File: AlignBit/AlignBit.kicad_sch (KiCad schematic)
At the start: 8 parts, among them J1 Conn_01x04_Pin, U1 STM32C011J_4-6_Mx, U4 VL53L0CXV0DH_1, U5 VL53L0CXV0DH_1, U6 VL53L0CXV0DH_1, U7 VL53L0CXV0DH_1

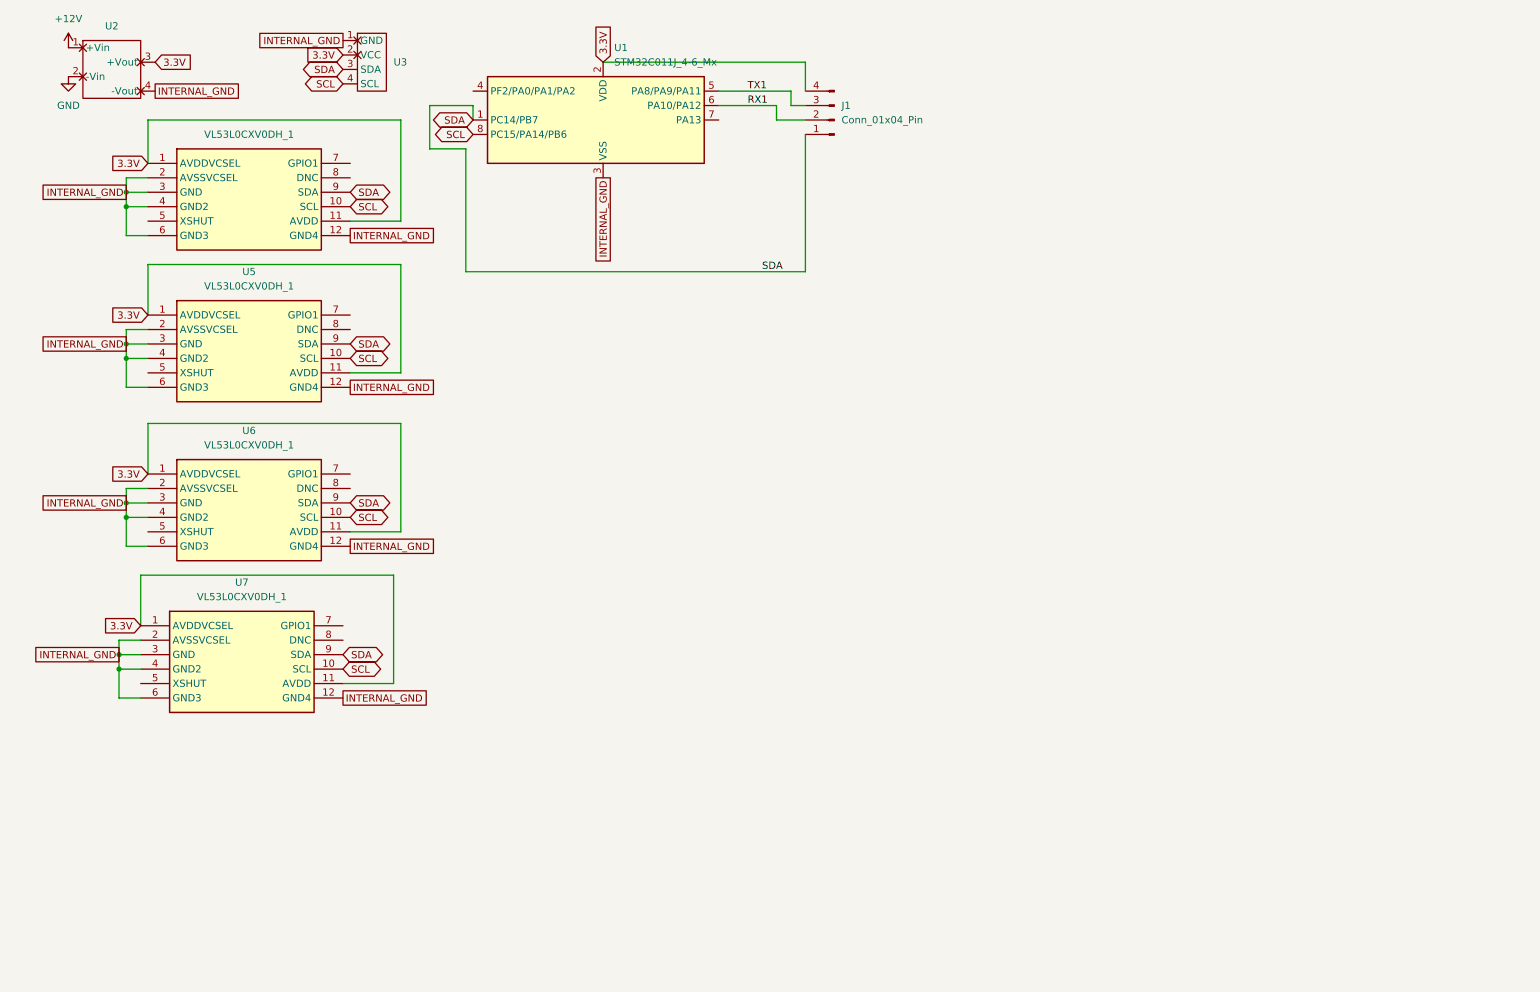
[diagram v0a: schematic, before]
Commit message: Adding things untill its done
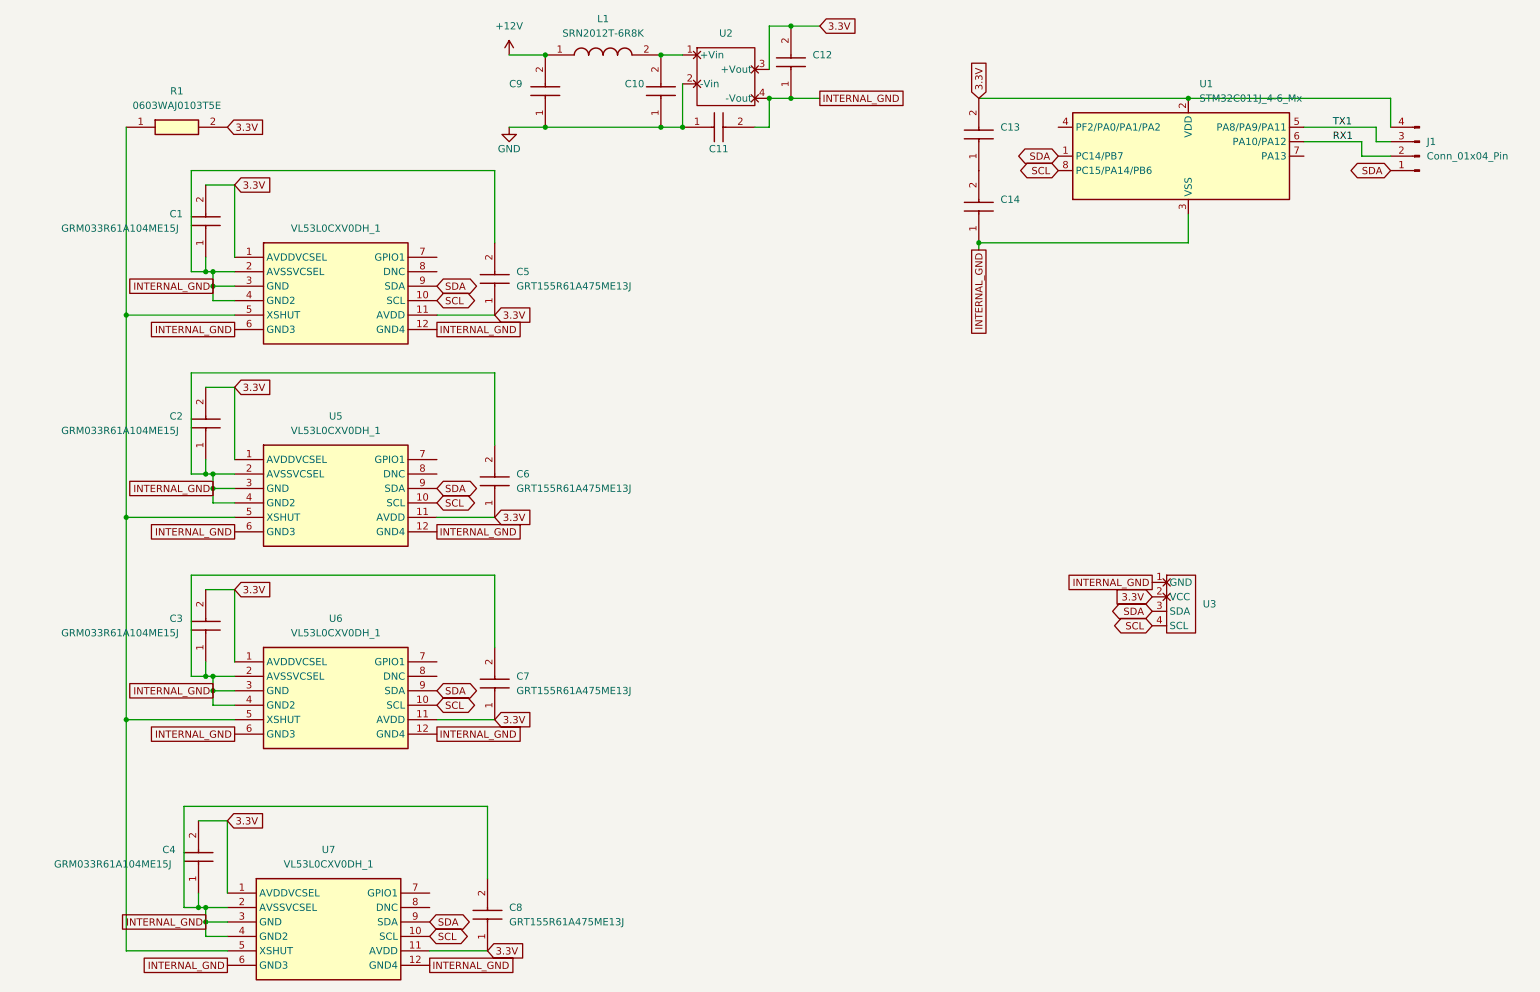
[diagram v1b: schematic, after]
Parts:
- added C1, C10, C13, C2, C3, C4, C9: GRM033R61A104ME15J, CAPC0603X33N, symbol GRM033R61A104ME15J:GRM033R61A104ME15J
- added C11: C0402C271K5RAC, CAPC1005X55N, symbol C0402C271K5RAC:C0402C271K5RAC
- added C12: GRM188R61C106MA73J, CAPC1608X90N, symbol GRM188R61C106MA73J:GRM188R61C106MA73J
- added C14, C5, C6, C7, C8: GRT155R61A475ME13J, CAPC1005X55N, symbol GRT155R61A475ME13J:GRT155R61A475ME13J
- added L1: SRN2012T-6R8K, INDPM2012X120N, symbol SRN2012T-6R8K:SRN2012T-6R8K
- added R1: 0603WAJ0103T5E, RESC1608X55N, symbol 0603WAJ0103T5E:0603WAJ0103T5E
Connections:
- net +12V: now also C9.2, L1.1; no longer U2.1 (+Vin)
- net 3.3V: now also C1.2, C12.2, C13.2, C2.2, C3.2, C4.2, C5.1, C6.1, C7.1, C8.1, R1.2
- net GND: now also C10.1, C11.1, C9.1
- net INTERNAL_GND: now also C1.1, C11.2, C12.1, C14.1, C2.1, C3.1, C4.1, C5.2, C6.2, C7.2, C8.2
- net at U4.5 (XSHUT): now also U5.5 (XSHUT), U6.5 (XSHUT), U7.5 (XSHUT), R1.1
- new net: C13.1, C14.2
- new net: C10.2, L1.2, U2.1 (+Vin)
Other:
- moved on the sheet: J1, U1, U2, U3, U5, U6, U7
